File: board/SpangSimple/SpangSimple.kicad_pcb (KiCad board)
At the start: 2 copper layers, 37.5 x 43.5 mm, 14 parts

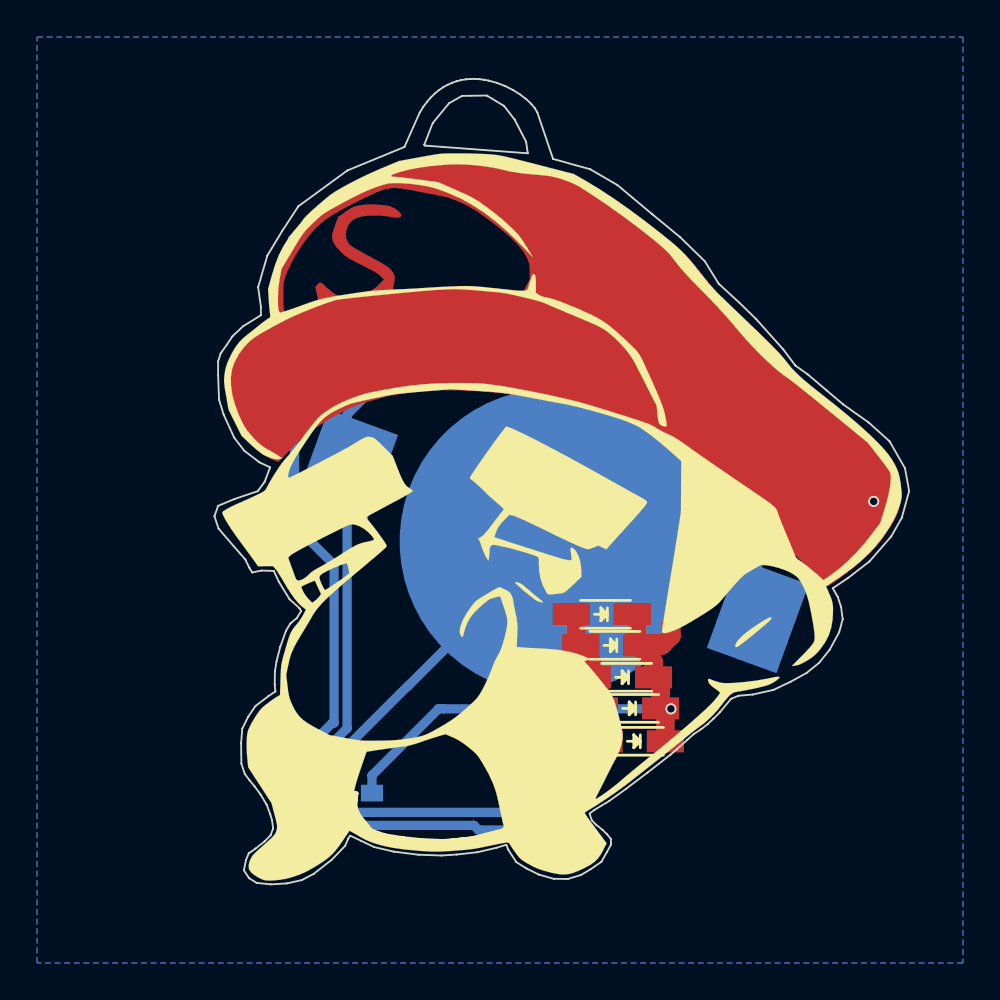
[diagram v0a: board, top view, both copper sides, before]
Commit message: kfdjkd
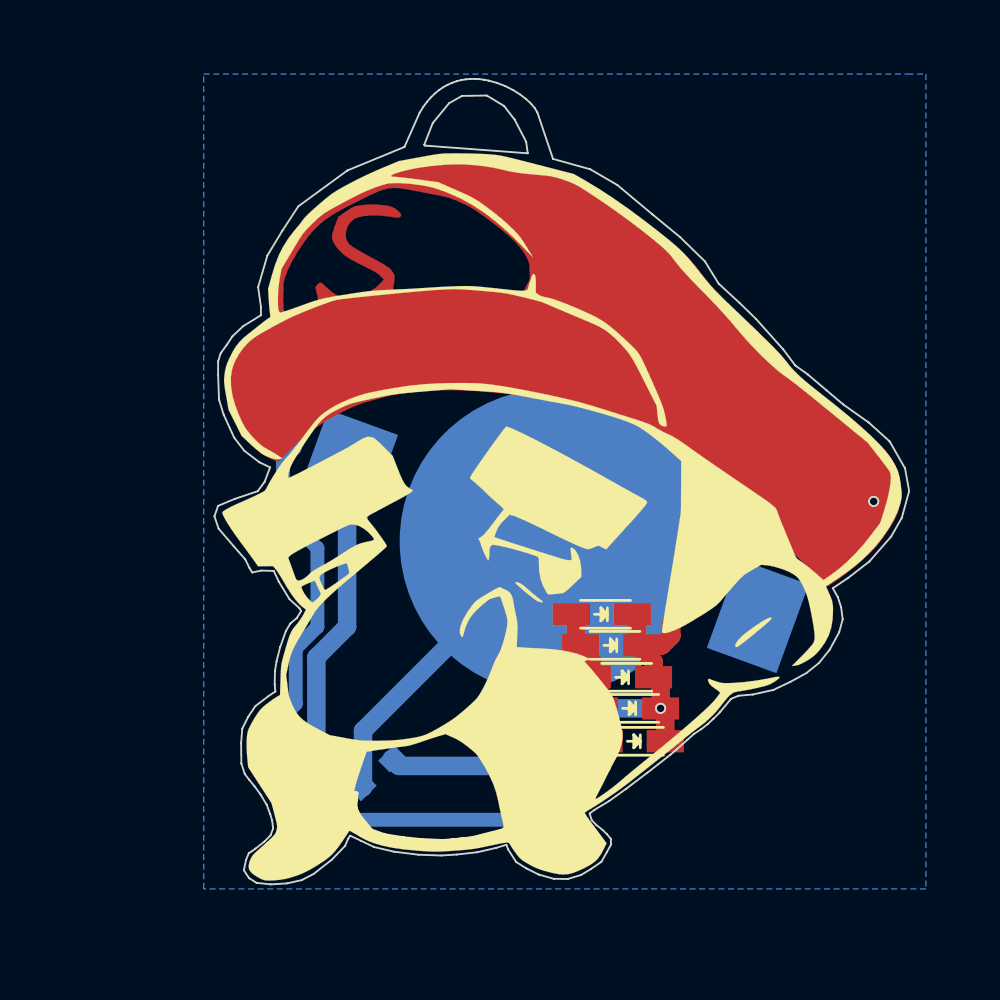
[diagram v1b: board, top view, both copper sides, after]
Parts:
- F1: value Fuse -> Polyfuse
- moved D6 12.8 mm to (139.2, 115.1), turned to 315 degrees
- moved D8 2.87 mm to (142.5, 90.0)
- moved F1 1.76 mm to (143.4, 114.8), turned to 225 degrees
- moved D7 0.24 mm to (148.2, 83.1), turned to 340 degrees
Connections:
- F1 pad 1: Net-(BT1-Pad2) -> GND
- F1 pad 2: GND -> Net-(BT1-Pad2)
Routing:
- net Net-(BT1-Pad1): track 69.9 -> 21.3 mm
- net Net-(BT1-Pad2): track 18.5 -> 29.4 mm
- net +BATT: track 72.6 -> 75.6 mm
- net Net-(D7-Pad1): track 42.9 -> 45.7 mm
- net GND: track 50.7 -> 48.5 mm
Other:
- board text added: "CC"
- board text added: "CC Attr. ShareAlike 4.0 Int."
- board text added: "REMOVE BATTERY WHEN NOT IN USE"
